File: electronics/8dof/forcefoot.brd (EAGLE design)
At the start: 120 x 32 mm, 121 parts

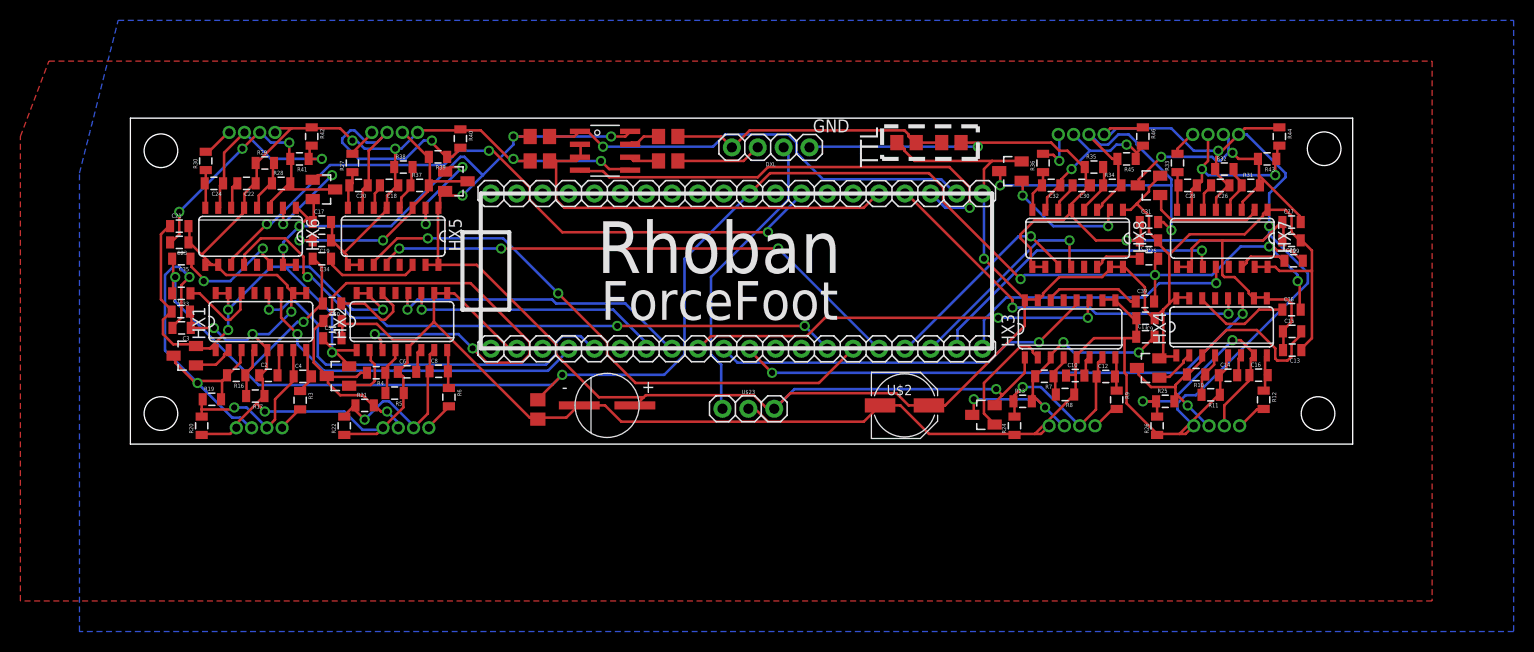
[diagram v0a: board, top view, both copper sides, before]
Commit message: Fix
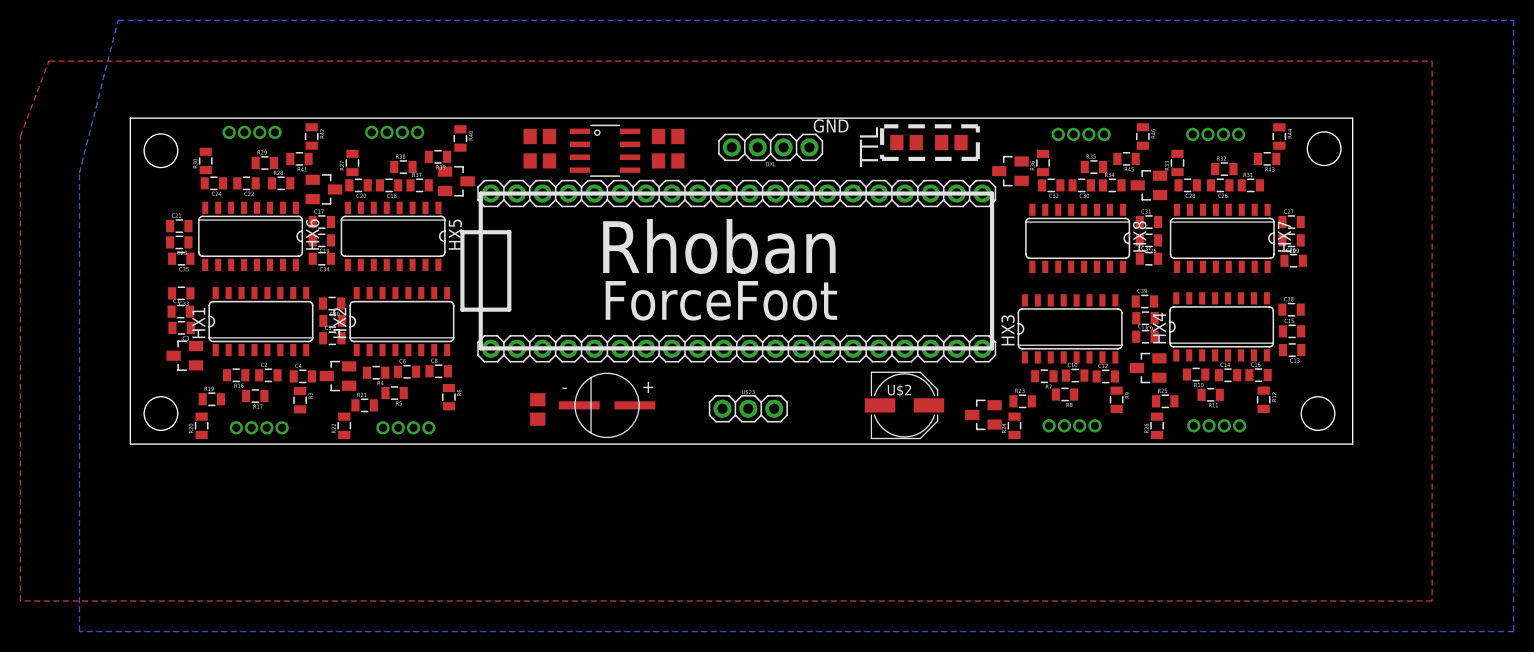
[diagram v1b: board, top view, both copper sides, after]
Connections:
- net DIRECTION: now also MAPLE_MINI.X2; no longer MAPLE_MINI.X3
- net DOUT4: now also MAPLE_MINI.X3; no longer MAPLE_MINI.X2
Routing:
- net GND: track 469.7 -> 0.00 mm, vias 12 -> 0
- net VCC: track 342.7 -> 0.00 mm, vias 11 -> 0
- net CLOCK: track 172.1 -> 0.00 mm, vias 7 -> 0
- net SCK5: track 67.0 -> 0.00 mm, vias 3 -> 0
- net AVDD$2: track 65.0 -> 0.00 mm, vias 3 -> 0
- net DOUT5: track 64.4 -> 0.00 mm, vias 3 -> 0
- net SCK6: track 56.4 -> 0.00 mm, vias 2 -> 0
- net SCK4: track 53.5 -> 0.00 mm, vias 2 -> 0
- net DOUT6: track 53.3 -> 0.00 mm, vias 3 -> 0
- net AVDD$7: track 46.6 -> 0.00 mm, vias 2 -> 0
- net TX: track 46.2 -> 0.00 mm, vias 1 -> 0
- net RX: track 44.3 -> 0.00 mm, vias 1 -> 0
- net SCK3: track 41.3 -> 0.00 mm, vias 2 -> 0
- net DIRECTION: track 40.9 -> 0.00 mm
- net DOUT1: track 40.8 -> 0.00 mm, vias 1 -> 0
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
